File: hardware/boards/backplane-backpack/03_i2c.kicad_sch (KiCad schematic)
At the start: 10 parts, among them J11 backplane_mate, U2 TCA9548APWR

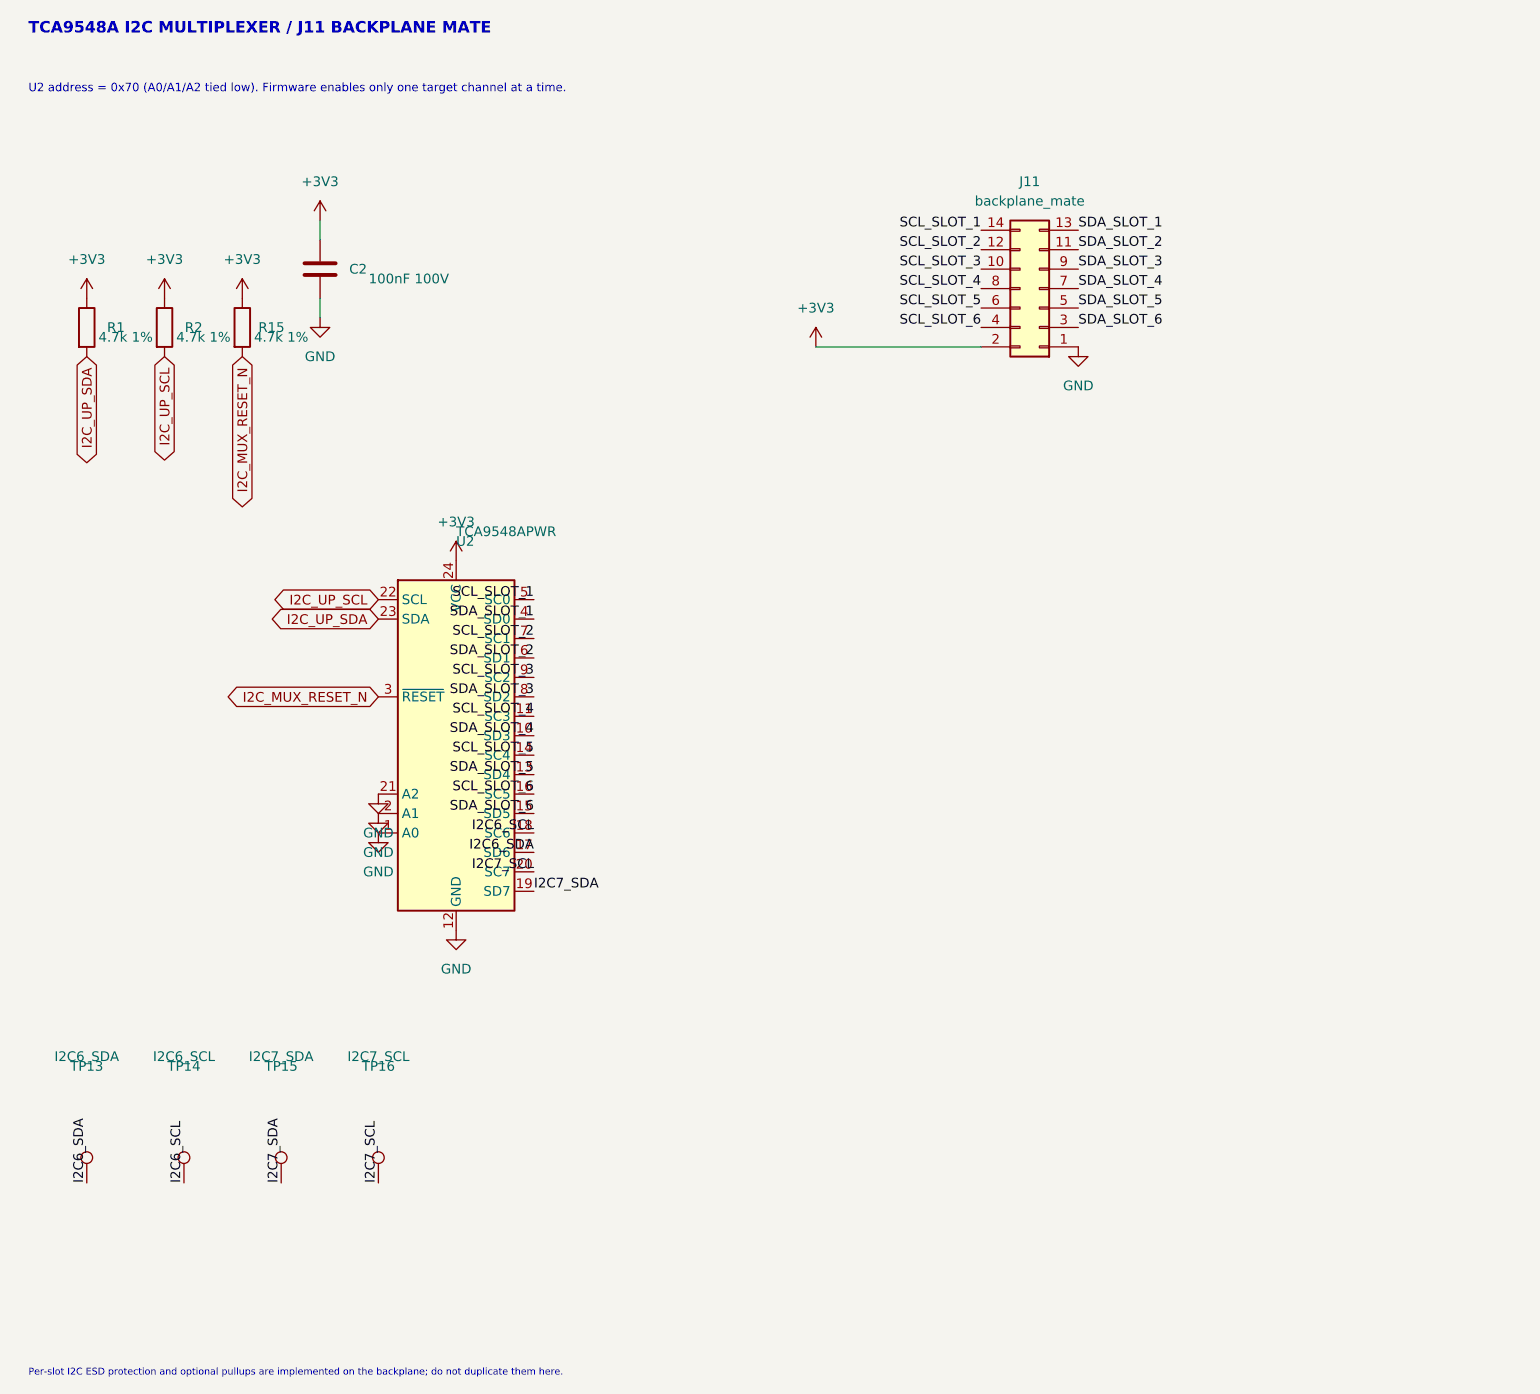
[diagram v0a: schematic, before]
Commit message: chore: checkpoint current design changes
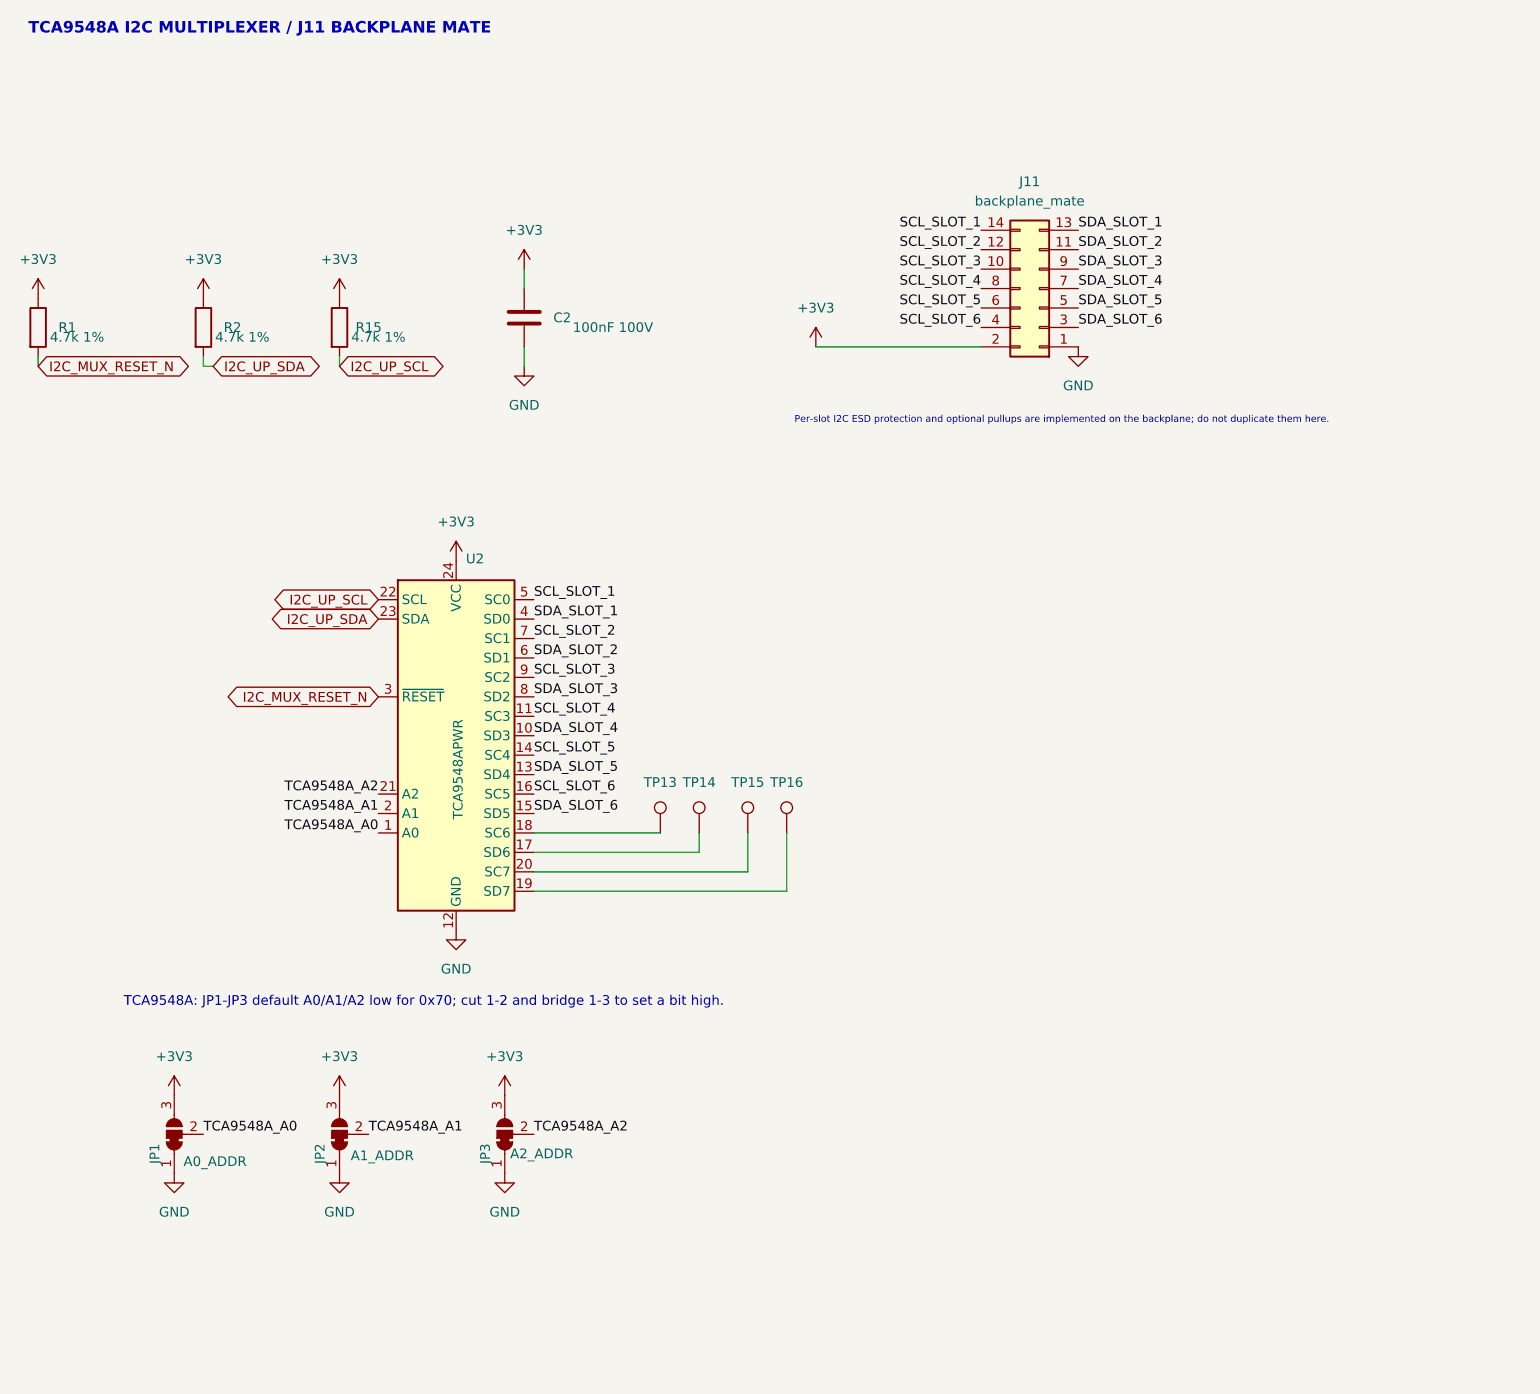
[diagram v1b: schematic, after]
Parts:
- added JP1: A0_ADDR, Jumper:SolderJumper-3_P1.3mm_Bridged12_Pad1.0x1.5mm, symbol Jumper:SolderJumper_3_Bridged12
- added JP2: A1_ADDR, Jumper:SolderJumper-3_P1.3mm_Bridged12_Pad1.0x1.5mm, symbol Jumper:SolderJumper_3_Bridged12
- added JP3: A2_ADDR, Jumper:SolderJumper-3_P1.3mm_Bridged12_Pad1.0x1.5mm, symbol Jumper:SolderJumper_3_Bridged12
- TP14: value I2C6_SCL -> I2C6_SDA
- TP15: value I2C7_SDA -> I2C6_SDA
- TP16: value I2C7_SCL -> I2C6_SDA
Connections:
- net +3V3: now also JP1.3 (B), JP2.3 (B), JP3.3 (B)
- net GND: now also JP1.1 (A), JP2.1 (A), JP3.1 (A); no longer U2.1 (A0), U2.2 (A1), U2.21 (A2)
- net I2C_MUX_RESET_N: now also R1.2; no longer R15.2
- net I2C_UP_SCL: now also R15.2; no longer R2.2
- net I2C_UP_SDA: now also R2.2; no longer R1.2
- net I2C6_SCL: no longer names the net of TP14.1
- net I2C6_SCL: now also U2.17 (SD6); no longer U2.18 (SC6)
- net I2C6_SDA: no longer names the net of TP13.1
- net I2C6_SDA: now also U2.18 (SC6); no longer U2.17 (SD6)
- net I2C7_SCL: no longer names the net of TP16.1
- net I2C7_SCL: now also U2.19 (SD7); no longer U2.20 (SC7)
- net I2C7_SDA: no longer names the net of TP15.1
- net I2C7_SDA: now also U2.20 (SC7); no longer U2.19 (SD7)
- new net TCA9548A_A0: JP1.2 (C), U2.1 (A0)
- new net TCA9548A_A1: JP2.2 (C), U2.2 (A1)
- new net TCA9548A_A2: JP3.2 (C), U2.21 (A2)
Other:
- note added: "TCA9548A: JP1-JP3 default A0/A1/A2 low for 0x70; cut 1-2 and bridge 1-3 to set a bit high."
- note removed: "U2 address = 0x70 (A0/A1/A2 tied low). Firmware enables only one target channel at a time."
- moved on the sheet: C2, R1, R15, R2, TP13
